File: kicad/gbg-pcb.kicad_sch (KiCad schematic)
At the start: 53 parts, among them IC2 D78B05T-1.0, J1 9 2.54mm pitch header pins, J12 screw terminal, J2 Conn_01x02, J3 VP0265840000G, J4 Screw_Terminal_01x04, J5 Screw_Terminal_01x03, J8 1017514, J9 1017514, P1 rpi pico, Q1 PSMN1R2-25YLDX, Q2 PSMN1R2-25YLDX, Q3 PSMN1R2-25YLDX, Q4 PSMN1R2-25YLDX, SW1 screw terminal, U1 IFX007TAUMA1, U2 IFX007TAUMA1, U3 IFX007TAUMA1, U4 IFX007TAUMA1

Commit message: v1.1
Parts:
- C3, C5: footprint Capacitor_THT:CP_Radial_D10.0mm_P7.50mm -> kicad libraries:CP_Radial_D10.0mm_P5.00mm
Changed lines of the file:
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@@
 			)
 		)
-		(property "Footprint" "Capacitor_THT:CP_Radial_D10.0mm_P7.50mm"
+		(property "Footprint" "kicad libraries:CP_Radial_D10.0mm_P5.00mm"
 			(at 216.8652 120.65 0)
 			(effects
@@
 			)
 		)
-		(property "Footprint" "Capacitor_THT:CP_Radial_D10.0mm_P7.50mm"
+		(property "Footprint" "kicad libraries:CP_Radial_D10.0mm_P5.00mm"
 			(at 204.1652 38.1 0)
 			(effects

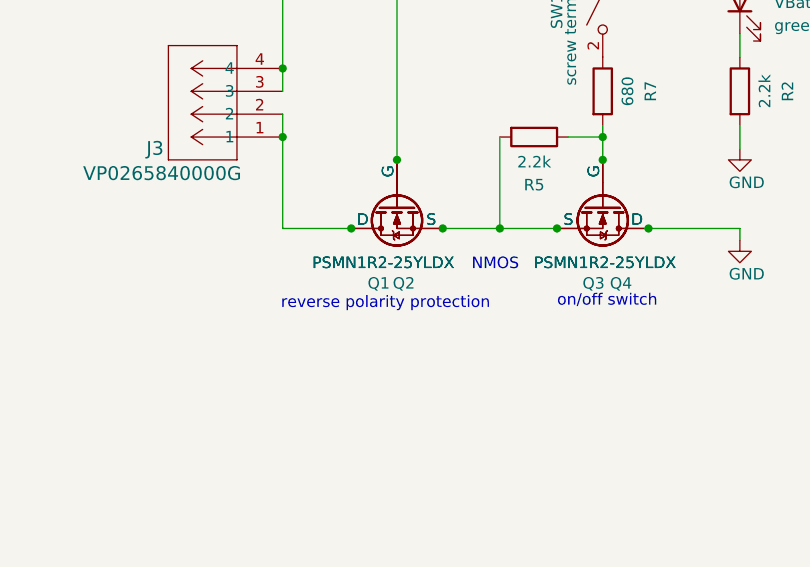
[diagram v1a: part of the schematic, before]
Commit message: adjust labels
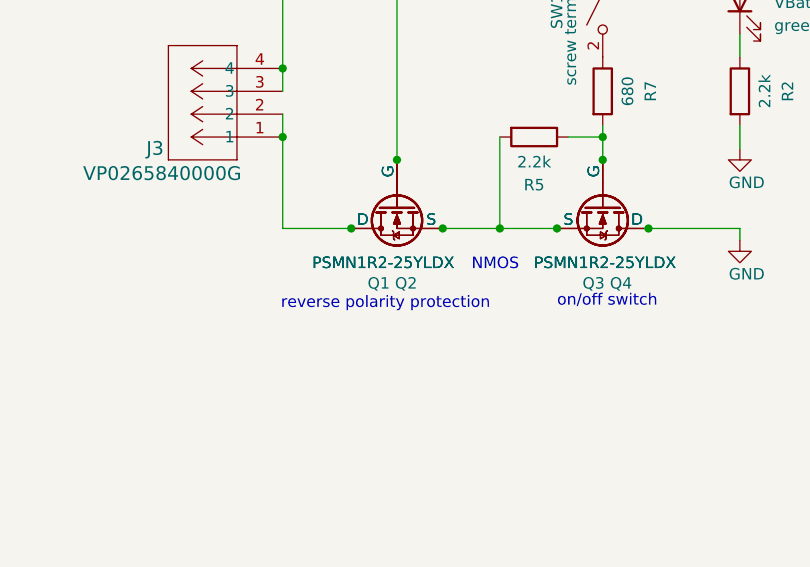
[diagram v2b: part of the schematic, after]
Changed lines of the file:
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@@
 		(dnp no)
 		(property "Reference" "Q2"
-			(at 150.622 242.316 90)
+			(at 150.876 242.316 90)
 			(effects
 				(font
